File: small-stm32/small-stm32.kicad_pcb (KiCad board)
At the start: 4 copper layers, 17.8 x 21 mm, 42 parts, among them J1 USB_C_Receptacle, J3 QWIIC, U2 STM32G0B1CBUxN, U3 SGM6029, Y1 8Mhz SMD2520-4P

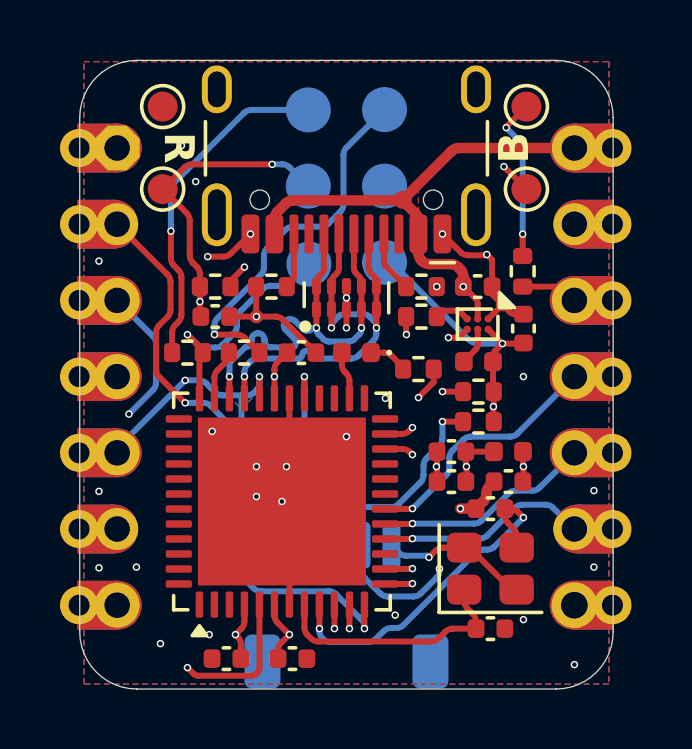
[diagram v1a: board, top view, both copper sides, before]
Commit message: .
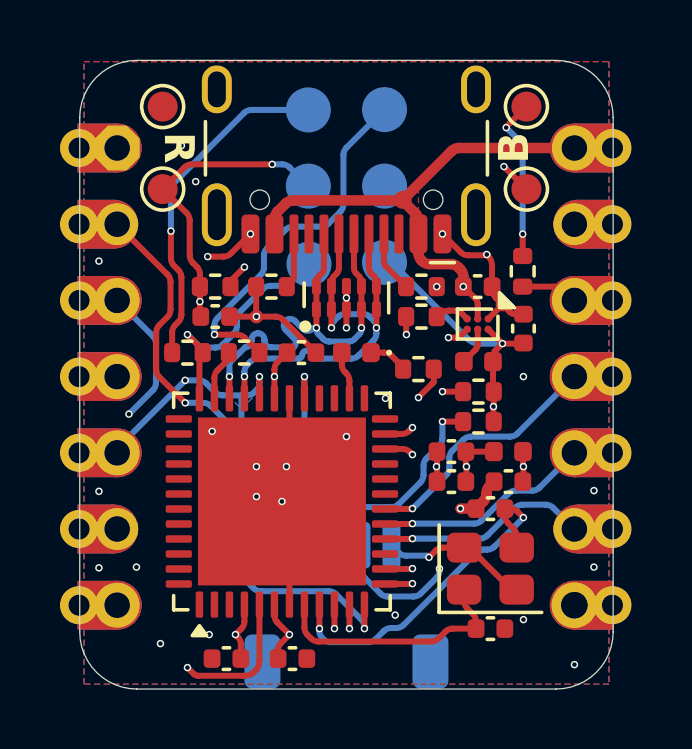
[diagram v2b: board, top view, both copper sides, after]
